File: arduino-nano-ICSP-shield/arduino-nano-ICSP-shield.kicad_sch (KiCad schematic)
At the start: 9 parts, among them J1 Analog, J2 Digital, J3 AVR-ISP-6, J4 Conn_02x04_Counter_Clockwise

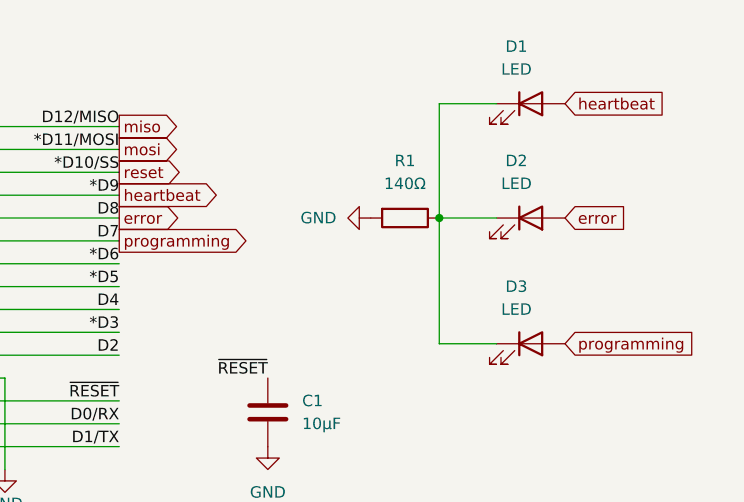
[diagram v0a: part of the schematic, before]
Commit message: flip resistor
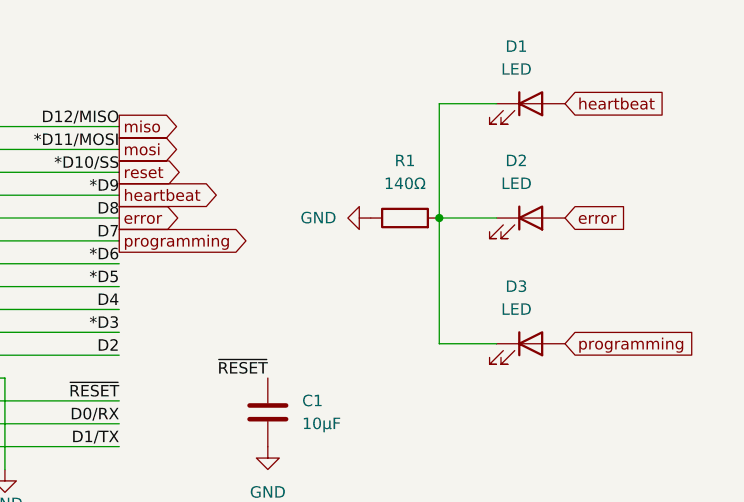
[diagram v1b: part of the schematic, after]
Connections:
- net GND: now also R1.1; no longer R1.2
- net at D1.1 (K), D2.1 (K), D3.1 (K): now also R1.2; no longer R1.1
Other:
- moved on the sheet: R1
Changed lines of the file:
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@@
 	(symbol
 		(lib_id "Device:R")
-		(at 102.87 36.83 270)
+		(at 102.87 36.83 90)
 		(unit 1)
 		(exclude_from_sim no)
@@
 		)
 		(property "Footprint" "Resistor_SMD:R_0603_1608Metric"
-			(at 102.87 35.052 90)
+			(at 102.87 38.608 90)
 			(effects
 				(font
